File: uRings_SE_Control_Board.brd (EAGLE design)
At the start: 40 x 110.5 mm, 27 parts, among them J1 JACK, J10 JACK, J2 JACK, J3 JACK, J4 JACK, J5 JACK, J6 JACK, J7 JACK, J8 JACK, J9 JACK, P1 B10k, P10 B10k, P2 B10k, P3 B10k, P4 B10k, P5 B10k, P6 B10k, P7 B10k, P8 B10k, P9 B10k

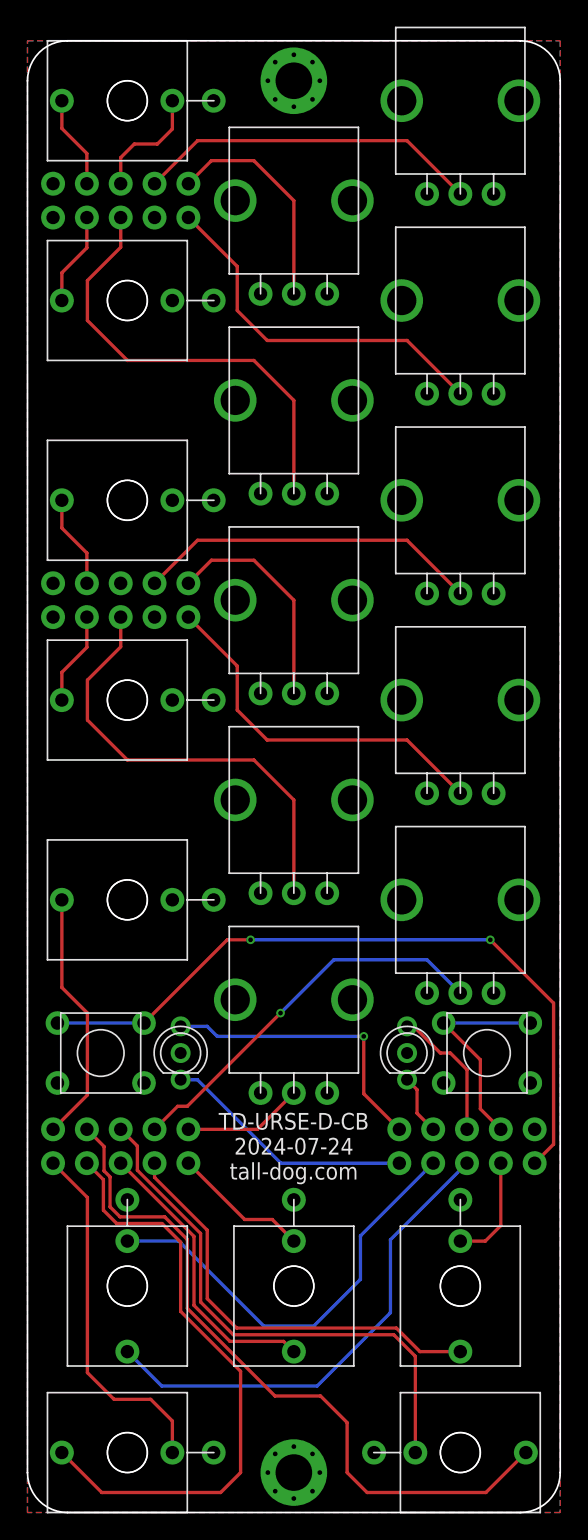
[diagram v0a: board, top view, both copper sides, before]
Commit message: revision D updates continued
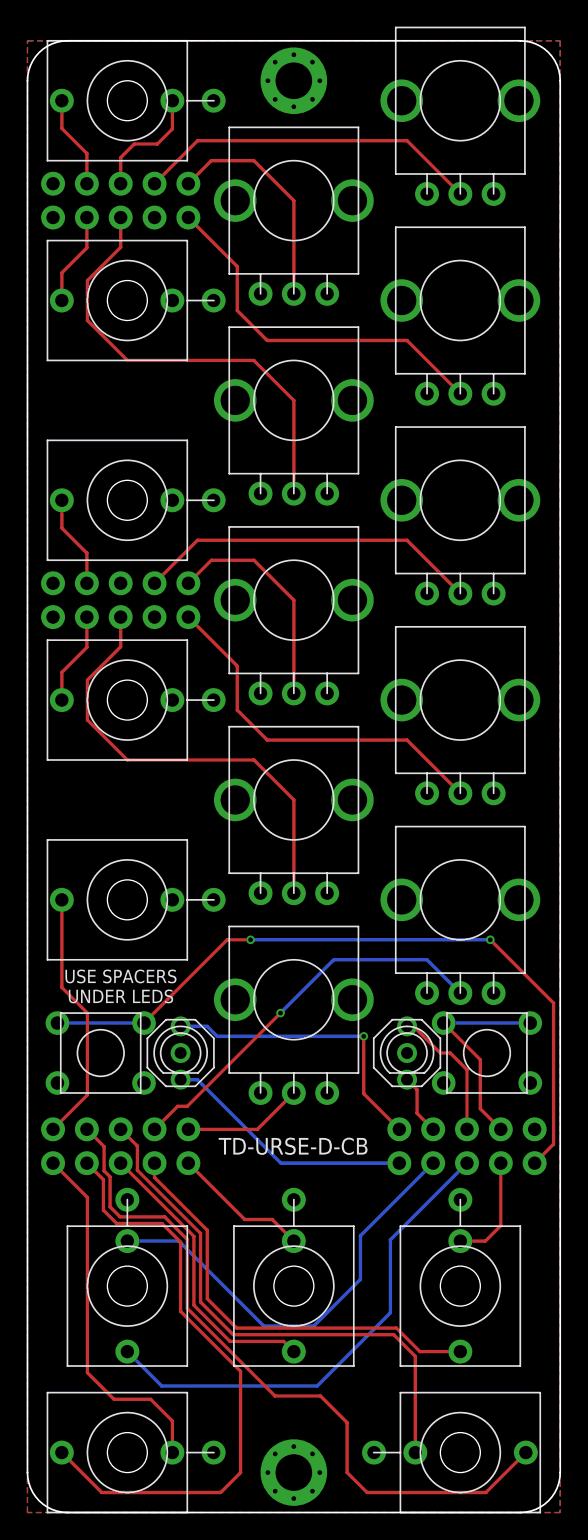
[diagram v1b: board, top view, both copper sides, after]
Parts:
- added U$1, U$2: (no value), uRings_SE_Library:LED-SPACER
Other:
- board text added: "2024-08-07"
- board text added: "CC BY-SA 4.0"
- board text added: "Control Board"
- board text added: "USE SPACERS UNDER LEDS"
- board text added: "µRings SE"
- board text removed: "2024-07-24"
- board text removed: "TD-URSE-D-CB 2024-07-24 tall-dog.com"
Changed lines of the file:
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@@
 <layer number="48" name="Document" color="7" fill="1" visible="no" active="yes"/>
 <layer number="49" name="Reference" color="7" fill="1" visible="no" active="yes"/>
-<layer number="51" name="tDocu" color="7" fill="1" visible="no" active="yes"/>
-<layer number="52" name="bDocu" color="7" fill="1" visible="yes" active="yes"/>
+<layer number="51" name="tDocu" color="48" fill="1" visible="no" active="yes"/>
+<layer number="52" name="bDocu" color="48" fill="1" visible="no" active="yes"/>
 <layer number="88" name="SimResults" color="9" fill="1" visible="no" active="no"/>
 <layer number="89" name="SimProbes" color="9" fill="1" visible="no" active="no"/>
@@
 <wire x1="40" y1="3" x2="37" y2="0" width="0.127" layer="20" curve="-90"/>
 <wire x1="37" y1="110.5" x2="40" y2="107.5" width="0.127" layer="20" curve="-90"/>
-<text x="20" y="57.5" size="1.5" layer="22" ratio="10" rot="MR0" align="center">TD-URSE-D-CB</text>
-<text x="20" y="49.5" size="1.5" layer="22" ratio="10" rot="MR0" align="center">2024-07-24</text>
-<text x="20" y="27.5" size="1.25" layer="21" ratio="10" align="center">TD-URSE-D-CB
-2024-07-24
-tall-dog.com</text>
+<text x="20" y="80" size="1.5" layer="22" ratio="10" rot="MR0" align="center">TD-URSE-D-CB</text>
+<text x="20" y="49.5" size="1.5" layer="22" ratio="10" rot="MR0" align="center">2024-08-07</text>
+<text x="20" y="27.5" size="1.25" layer="21" ratio="10" align="center">TD-URSE-D-CB</text>
 <text x="20" y="42.5" size="1.5" layer="22" ratio="10" rot="MR0" align="center">tall-dog.com</text>
 <text x="7" y="98.5" size="1" layer="52" ratio="10" rot="MR0" align="center">H1</text>
@@
 <text x="13.75" y="27.5" size="1" layer="22" ratio="10" rot="MR90" align="bottom-center">H3</text>
 <text x="26.25" y="27.5" size="1" layer="22" ratio="10" rot="MR270" align="bottom-center">H4</text>
+<text x="7" y="39.5" size="1" layer="21" ratio="10" align="center">USE SPACERS
+UNDER LEDS</text>
+<text x="20" y="30.5" size="1" layer="51" ratio="10" align="center">USE SPACERS UNDER LEDS</text>
+<text x="19.5" y="87.5" size="1.5" layer="22" ratio="10" rot="MR0" align="center">Control Board</text>
+<text x="19.5" y="95" size="1.5" layer="22" ratio="10" rot="MR0" align="center">µRings SE</text>
+<text x="20" y="57.5" size="1.5" layer="22" ratio="10" rot="MR0" align="center">CC BY-SA 4.0</text>
 </plain>
 <attributes>
@@
 <element name="J10" library="uRings_SE_Library" package="JACK" value="JACK" x="32.5" y="4.5" smashed="yes" rot="R270">
 <attribute name="NAME" x="27.5" y="9" size="1" layer="21" ratio="10" align="top-right"/>
-<attribute name="NAME" x="36.25" y="4.5" size="1" layer="51" ratio="10" rot="R270" align="center"/>
+<attribute name="NAME" x="32.5" y="4.5" size="1" layer="51" ratio="10" rot="R270" align="center"/>
 </element>
 <element name="J1" library="uRings_SE_Library" package="JACK" value="JACK" x="7.5" y="106" smashed="yes" rot="R90">
 <attribute name="NAME" x="12.5" y="110" size="1" layer="21" ratio="10" rot="R180" align="bottom-right"/>
-<attribute name="NAME" x="3.75" y="106" size="1" layer="51" ratio="10" rot="R90" align="center"/>
+<attribute name="NAME" x="7.5" y="106" size="1" layer="51" ratio="10" rot="R90" align="center"/>
 </element>
 <element name="J9" library="uRings_SE_Library" package="JACK" value="JACK" x="7.5" y="4.5" smashed="yes" rot="R90">
 <attribute name="NAME" x="12.5" y="9" size="1" layer="21" ratio="10" rot="R180" align="bottom-right"/>
-<attribute name="NAME" x="3.75" y="4.5" size="1" layer="51" ratio="10" rot="R90" align="center"/>
+<attribute name="NAME" x="7.5" y="4.5" size="1" layer="51" ratio="10" rot="R90" align="center"/>
 </element>
 <element name="J8" library="uRings_SE_Library" package="JACK" value="JACK" x="32.5" y="17" smashed="yes" rot="R180">
 <attribute name="NAME" x="28" y="22" size="1" layer="21" ratio="10"/>
-<attribute name="NAME" x="32.5" y="13.25" size="1" layer="51" ratio="10" rot="R180" align="center"/>
+<attribute name="NAME" x="32.5" y="17" size="1" layer="51" ratio="10" rot="R180" align="center"/>
 </element>
 <element name="J7" library="uRings_SE_Library" package="JACK" value="JACK" x="20" y="17" smashed="yes" rot="R180">
 <attribute name="NAME" x="15.5" y="22" size="1" layer="21" ratio="10"/>
-<attribute name="NAME" x="20" y="13.25" size="1" layer="51" ratio="10" rot="R180" align="center"/>
+<attribute name="NAME" x="20" y="17" size="1" layer="51" ratio="10" rot="R180" align="center"/>
 </element>
 <element name="J6" library="uRings_SE_Library" package="JACK" value="JACK" x="7.5" y="17" smashed="yes" rot="R180">
 <attribute name="NAME" x="3" y="22" size="1" layer="21" ratio="10"/>
-<attribute name="NAME" x="7.5" y="13.25" size="1" layer="51" ratio="10" rot="R180" align="center"/>
+<attribute name="NAME" x="7.5" y="17" size="1" layer="51" ratio="10" rot="R180" align="center"/>
 </element>
 <element name="J5" library="uRings_SE_Library" package="JACK" value="JACK" x="7.5" y="46" smashed="yes" rot="R90">
 <attribute name="NAME" x="12.5" y="50.5" size="1" layer="21" ratio="10" rot="R180" align="bottom-right"/>
-<attribute name="NAME" x="3.75" y="46" size="1" layer="51" ratio="10" rot="R90" align="center"/>
+<attribute name="NAME" x="7.5" y="46" size="1" layer="51" ratio="10" rot="R90" align="center"/>
 </element>
 <element name="J4" library="uRings_SE_Library" package="JACK" value="JACK" x="7.5" y="61" smashed="yes" rot="R90">
 <attribute name="NAME" x="12.5" y="65.5" size="1" layer="21" ratio="10" rot="R180" align="bottom-right"/>
-<attribute name="NAME" x="3.75" y="61" size="1" layer="51" ratio="10" rot="R90" align="center"/>
+<attribute name="NAME" x="7.5" y="61" size="1" layer="51" ratio="10" rot="R90" align="center"/>
 </element>
 <element name="J3" library="uRings_SE_Library" package="JACK" value="JACK" x="7.5" y="76" smashed="yes" rot="R90">
 <attribute name="NAME" x="12.5" y="80.5" size="1" layer="21" ratio="10" rot="R180" align="bottom-right"/>
-<attribute name="NAME" x="3.75" y="76" size="1" layer="51" ratio="10" rot="R90" align="center"/>
+<attribute name="NAME" x="7.5" y="76" size="1" layer="51" ratio="10" rot="R90" align="center"/>
 </element>
 <element name="J2" library="uRings_SE_Library" package="JACK" value="JACK" x="7.5" y="91" smashed="yes" rot="R90">
 <attribute name="NAME" x="12.5" y="95.5" size="1" layer="21" ratio="10" rot="R180" align="bottom-right"/>
-<attribute name="NAME" x="3.75" y="91" size="1" layer="51" ratio="10" rot="R90" align="center"/>
+<attribute name="NAME" x="7.5" y="91" size="1" layer="51" ratio="10" rot="R90" align="center"/>
 </element>
 <element name="P9" library="uRings_SE_Library" package="POT" value="B10k" x="32.5" y="46" smashed="yes" rot="R180">
@@
 </element>
 <element name="H1-H4" library="uRings_SE_Library" package="HEADERS-MALE" value="HEADERS-MALE" x="0" y="0" smashed="yes"/>
+<element name="U$1" library="uRings_SE_Library" package="LED-SPACER" value="" x="11.5" y="34.5" smashed="yes"/>
+<element name="U$2" library="uRings_SE_Library" package="LED-SPACER" value="" x="28.5" y="34.5" smashed="yes"/>
 </elements>
 <signals>
